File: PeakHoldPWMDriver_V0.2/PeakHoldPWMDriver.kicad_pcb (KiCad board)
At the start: 2 copper layers, 100.1 x 50 mm, 81 parts, among them J1 Screw_Terminal_01x06, J2 Screw_Terminal_01x08, J3 Mounting 3mm, J4 Mounting 3mm, J5 Mounting 3mm, J6 Mounting 3mm, Q1 AO3400, Q10 AO3400, Q11 AO3422, Q12 AO3422, Q13 AO3401A, Q14 BSP78, Q15 AO3401A, Q16 BSP78, Q2 AO3400, Q3 AO3422, Q4 AO3422, Q5 AO3401A, Q6 AO3401A, Q7 BSP78, Q8 BSP78, Q9 AO3400, U1 74LS32, U2 LM2901, U3 74LS74, U4 LTC6992, U5 74LS74, U6 LM78M05_TO220, U7 74LS08, U8 74LS08

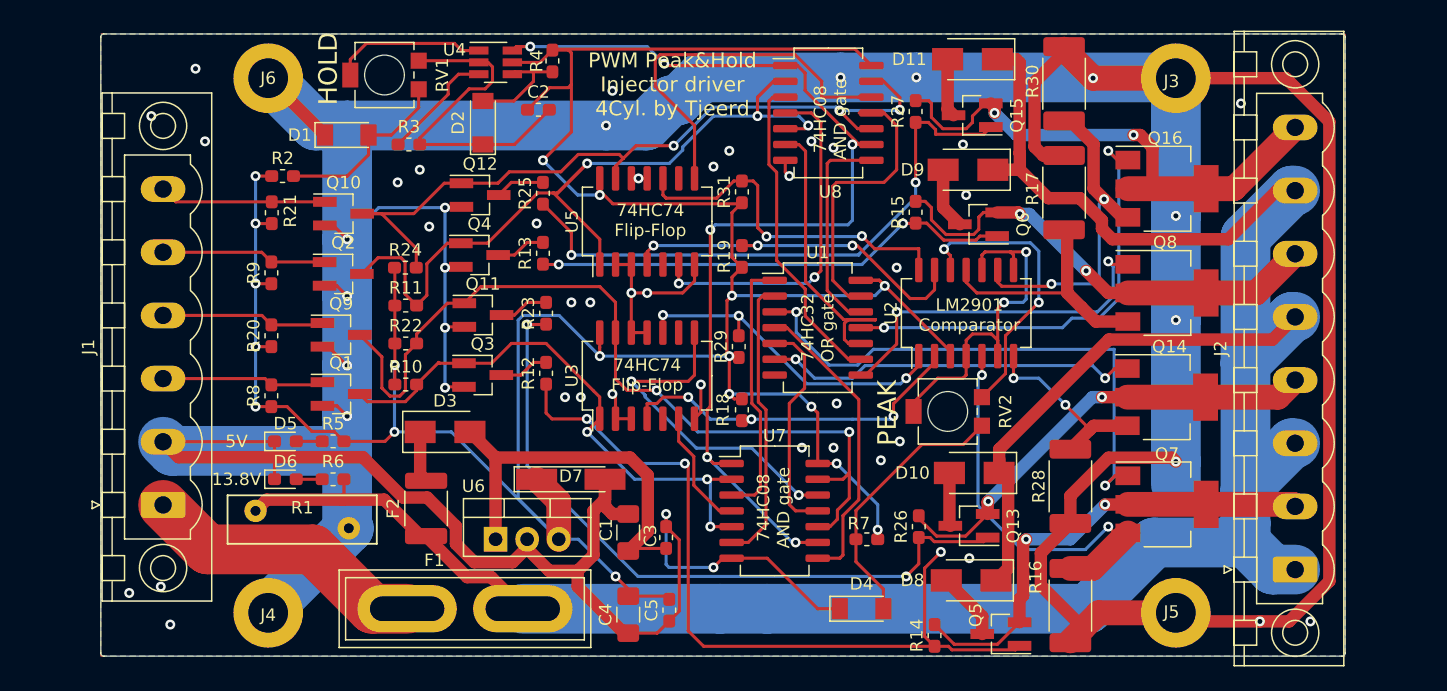
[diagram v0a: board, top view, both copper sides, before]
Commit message: Routing board V0.2
Work done on new PCB
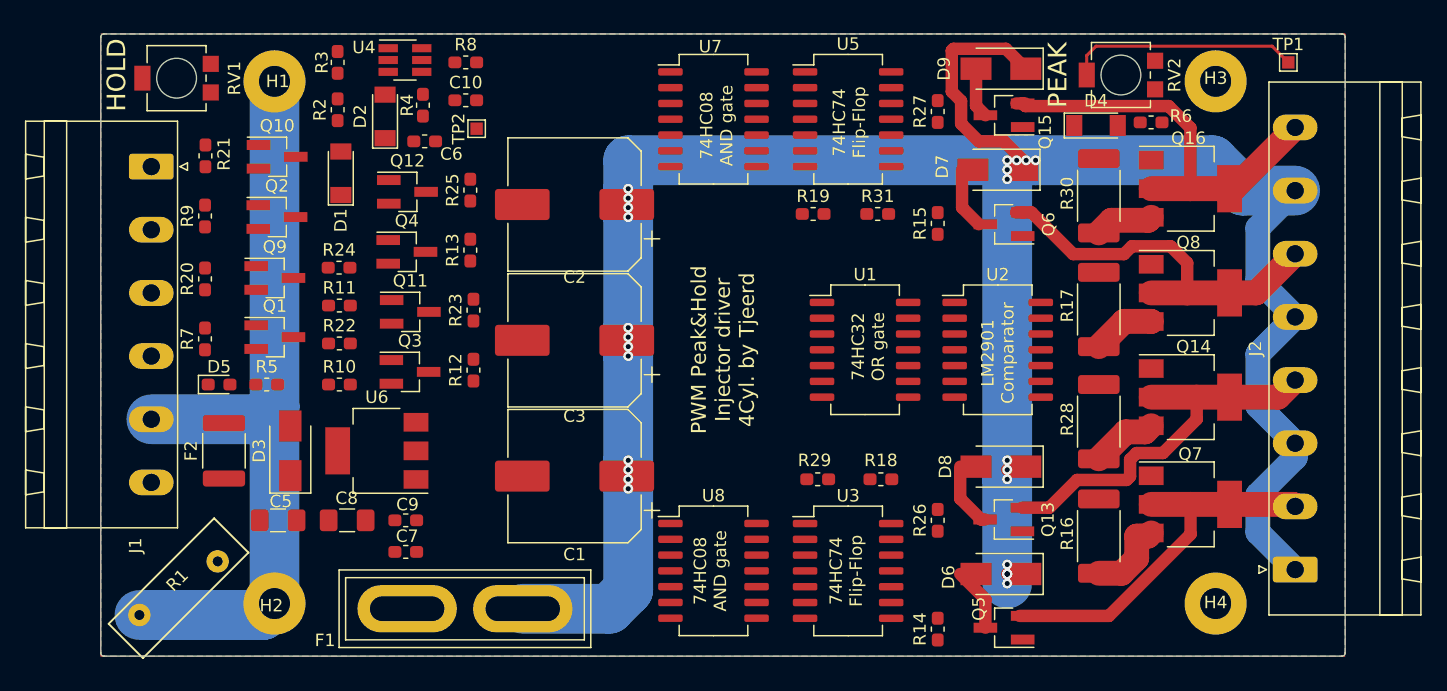
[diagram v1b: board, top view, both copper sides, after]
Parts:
- removed the D6 at (126.6, 101.9)
- removed the D7 at (149.6, 101.9)
- removed J3, J4, J5, J6: Mounting 3mm, MountingHole:MountingHole_3.2mm_M3_DIN965_Pad
- removed the R6 at (130.4, 101.9)
- removed the U7 at (166.0, 104.4)
- added C1: SVPF 1,0M 16, Capacitor_SMD:CP_Elec_10x12.5, F.Cu at (149.9, 101.6)
- added C10: 220nf, Capacitor_SMD:C_0603_1608Metric_Pad1.05x0.95mm_HandSolder, F.Cu at (141.1, 71.4)
- added C2: SVPF 1,0M 16, Capacitor_SMD:CP_Elec_10x12.5, F.Cu at (149.9, 79.8)
- added C3: SVPF 1,0M 16, Capacitor_SMD:CP_Elec_10x12.5, F.Cu at (149.9, 90.7)
- added H1: MountingHole_Pad, MountingHole:MountingHole_2.5mm_Pad, F.Cu at (125.7, 69.8)
- added H2: MountingHole_Pad, MountingHole:MountingHole_2.5mm_Pad, F.Cu at (125.7, 111.8)
- added H3: MountingHole_Pad, MountingHole:MountingHole_2.5mm_Pad, F.Cu at (201.4, 69.8)
- added H4: MountingHole_Pad, MountingHole:MountingHole_2.5mm_Pad, F.Cu at (201.4, 111.8)
- added R8: 8K2, Resistor_SMD:R_0603_1608Metric_Pad1.05x0.95mm_HandSolder, F.Cu at (141.1, 68.3)
- added TP1: PeakTP, TestPoint:TestPoint_Pad_1.0x1.0mm, F.Cu at (207.3, 68.3)
- added TP2: HoldTP, TestPoint:TestPoint_Pad_1.0x1.0mm, F.Cu at (142.0, 73.7)
- added U8: 74LS08, Package_SO:SO-14_5.3x10.2mm_P1.27mm, F.Cu at (161.0, 109.2)
- D1, D4: value LL4148 -> BAV103
- D3: value 40V-1A -> 1N4007
- D6: renamed from D8; value SS310 -> 1N4007
- D7: renamed from D9; value SS310 -> 1N4007
- D8: renamed from D10; value SS310 -> 1N4007
- D9: renamed from D11; value SS310 -> 1N4007
- J1: footprint Connector_Phoenix_MSTB:PhoenixContact_MSTBV_2,5_6-GF-5,08_1x06_P5.08mm_Vertical_ThreadedFlange -> Connector_Phoenix_MSTB:PhoenixContact_MSTBA_2,5_6-G-5,08_1x06_P5.08mm_Horizontal
- J2: footprint Connector_Phoenix_MSTB:PhoenixContact_MSTBV_2,5_8-GF-5,08_1x08_P5.08mm_Vertical_ThreadedFlange -> Connector_Phoenix_MSTB:PhoenixContact_MSTBA_2,5_8-G-5,08_1x08_P5.08mm_Horizontal
- Q11, Q12, Q3, Q4: value AO3422 -> 2N7002
- Q13, Q15, Q5, Q6: value AO3401A -> TSM2309
- U6: footprint Package_TO_SOT_THT:TO-220-3_Vertical -> Package_TO_SOT_SMD:SOT-223-3_TabPin2
- moved D4 43.2 mm to (191.8, 73.4)
- moved R6 40.6 mm to (196.2, 73.2)
- moved RV2 30.4 mm to (193.8, 69.3)
- moved C5 28.2 mm to (126.0, 105.2), turned to 180 degrees
- moved J1 27.2 mm to (115.8, 76.7), turned to 270 degrees
- moved C8 23.8 mm to (131.6, 105.2), turned to 0 degrees
- moved U3 22.5 mm to (171.9, 109.2), turned to 0 degrees
- moved C9 22.4 mm to (136.3, 105.2), turned to 0 degrees
- moved C7 21.0 mm to (136.3, 107.7), turned to 0 degrees
- moved R1 18.2 mm to (114.9, 112.8), turned to 45 degrees
- moved U5 18.1 mm to (171.9, 72.9), turned to 0 degrees
- moved F2 16.9 mm to (121.7, 99.6)
- moved RV1 16.7 mm to (117.9, 69.6)
- moved D3 12.5 mm to (127.0, 99.6), turned to 90 degrees
- moved R18 12.5 mm to (174.5, 101.9), turned to 0 degrees
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- renumbered C1 to C5, C2 to C6, C3 to C7, C4 to C8, C5 to C9, R7 to R6, R8 to R7, U8 to U7
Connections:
- C5 pad 2: Net-(C1-Pad2) -> Net-(C5-Pad2)
- C7 pad 2: Net-(C1-Pad2) -> Net-(C5-Pad2)
- D3 pad 1: Net-(D3-Pad1) -> Net-(C5-Pad2)
- D3 pad 2: Net-(C1-Pad2) -> Net-(D3-Pad2)
- F2 pad 2: Net-(D3-Pad1) -> Net-(D3-Pad2)
- J1 pad 1: VBAT_IN -> INJ4
- J1 pad 2: PWR_GND -> INJ3
- J1 pad 3: INJ1 -> INJ2
- J1 pad 4: INJ2 -> INJ1
- J1 pad 5: INJ3 -> PWR_GND
- J1 pad 6: INJ4 -> VBAT_IN
- U2 pad 10: VREF -> Net-(Q16-Pad3)
- U2 pad 11: Net-(Q8-Pad3) -> VREF
- U2 pad 13: Net-(R19-Pad2) -> Net-(R31-Pad2)
- U2 pad 14: Net-(R31-Pad2) -> Net-(R19-Pad2)
- U2 pad 4: VREF -> Net-(Q7-Pad3)
- U2 pad 5: Net-(Q7-Pad3) -> VREF
- U2 pad 6: VREF -> Net-(Q14-Pad3)
- U2 pad 7: Net-(Q14-Pad3) -> VREF
- U2 pad 8: VREF -> Net-(Q8-Pad3)
- U2 pad 9: Net-(Q16-Pad3) -> VREF
- U6 pad 1: Net-(C1-Pad2) -> Net-(C5-Pad2)
- U7 pad 10: inv_INJ4 -> inv_INJ3
- U7 pad 11: Net-(U1-Pad13) -> Net-(U1-Pad10)
- U7 pad 12: Net-(U5-Pad8) -> Net-(U5-Pad6)
- U7 pad 13: inv_INJ4 -> inv_INJ3
- U7 pad 2: inv_INJ3 -> inv_INJ1
- U7 pad 3: Net-(U1-Pad9) -> Net-(U1-Pad1)
- U7 pad 4: Net-(U5-Pad6) -> Net-(U5-Pad8)
- U7 pad 5: inv_INJ3 -> inv_INJ4
- U7 pad 6: Net-(U1-Pad10) -> Net-(U1-Pad13)
- U7 pad 8: Net-(U1-Pad12) -> Net-(U1-Pad9)
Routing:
- net PWR_GND: track 509.7 -> 63.6 mm, vias 56 -> 0
- net 5V: track 253.7 -> 0.00 mm, vias 18 -> 0
- net PWM: track 84.8 -> 0.00 mm, vias 6 -> 0
- net inv_INJ2: track 70.8 -> 0.00 mm, vias 2 -> 0
- net Net-(Q5-Pad1): track 64.8 -> 0.00 mm, vias 3 -> 0
- net inv_INJ3: track 64.8 -> 0.00 mm, vias 3 -> 0
- net inv_INJ4: track 63.4 -> 0.00 mm, vias 3 -> 0
- net Net-(Q13-Pad1): track 56.4 -> 0.00 mm, vias 2 -> 0
- net Net-(Q15-Pad1): track 47.6 -> 0.00 mm, vias 2 -> 0
- net inv_INJ1: track 46.0 -> 0.00 mm, vias 3 -> 0
- net Net-(Q7-Pad1): track 44.0 -> 0.00 mm, vias 2 -> 0
- net Net-(Q6-Pad1): track 38.6 -> 0.00 mm, vias 2 -> 0
- net Net-(Q16-Pad1): track 36.3 -> 0.00 mm, vias 2 -> 0
- net Net-(C1-Pad2): track 32.2 -> 0.00 mm
- net Net-(U5-Pad8): track 31.6 -> 0.00 mm
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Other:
- board text removed: "13.8V"
- board text removed: "5V"
